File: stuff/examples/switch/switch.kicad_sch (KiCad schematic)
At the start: 12 parts

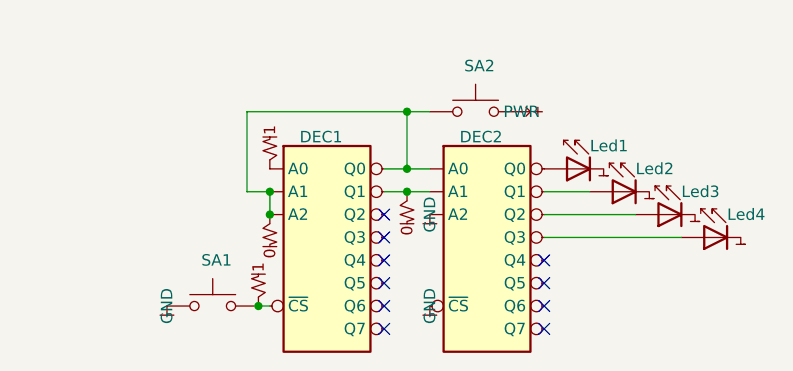
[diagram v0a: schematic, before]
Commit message: model build fixes
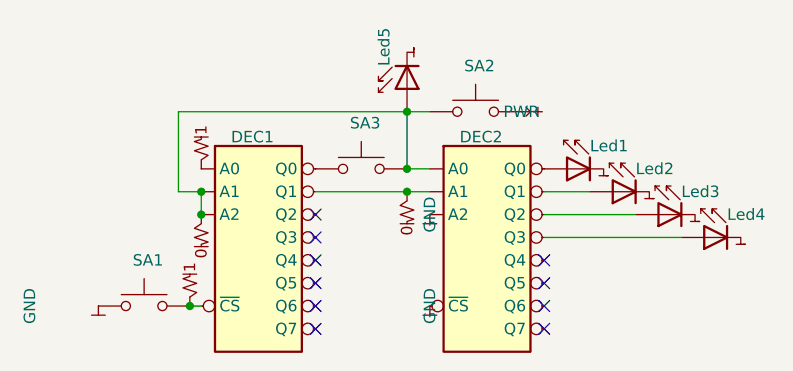
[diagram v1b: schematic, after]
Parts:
- added Led5: ~, symbol chip:LED
- added SA3: SW_Push, symbol Switch:SW_Push
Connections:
- net at DEC1.2 (A1), DEC1.3 (A2), DEC2.1 (A0)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: now also Led5.1 (IN), SA3.2; no longer DEC1.4 (Q0)
- new net: DEC1.4 (Q0), SA3.1
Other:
- moved on the sheet: DEC1, SA1
